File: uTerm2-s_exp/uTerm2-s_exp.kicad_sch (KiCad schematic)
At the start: 17 parts, among them J1 Conn_01x16_Female, J2 USB_B_Mini, J3 SD_Card, J4 Conn_01x08_Female, U1 ESP-PSRAM32, U2 CH340G, Y1 12MHz

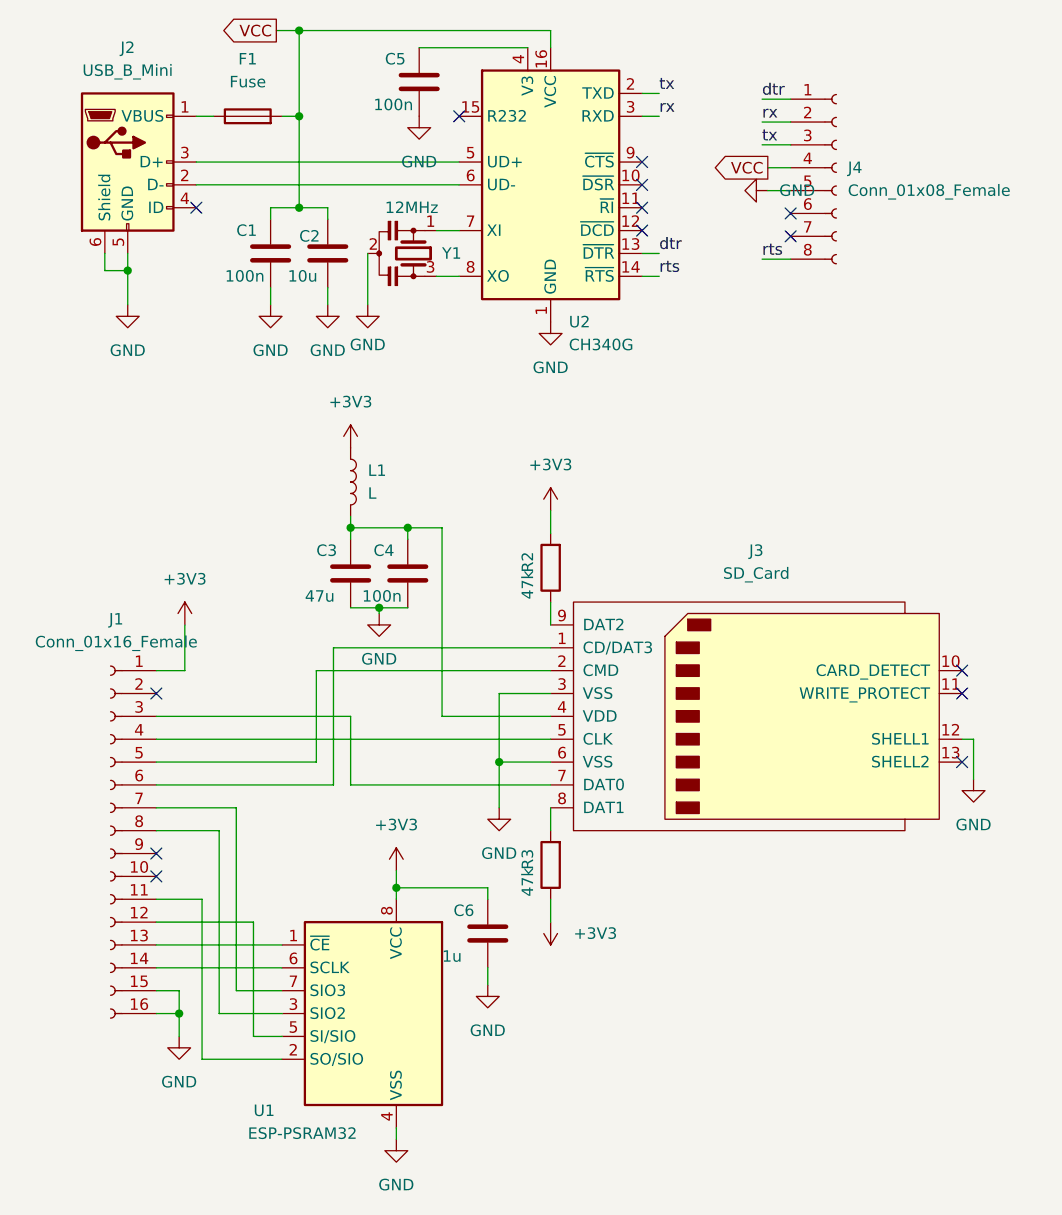
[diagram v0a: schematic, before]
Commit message: Signed-off-by: DamianPodrazaCode <damian.podraza@gmail.com>
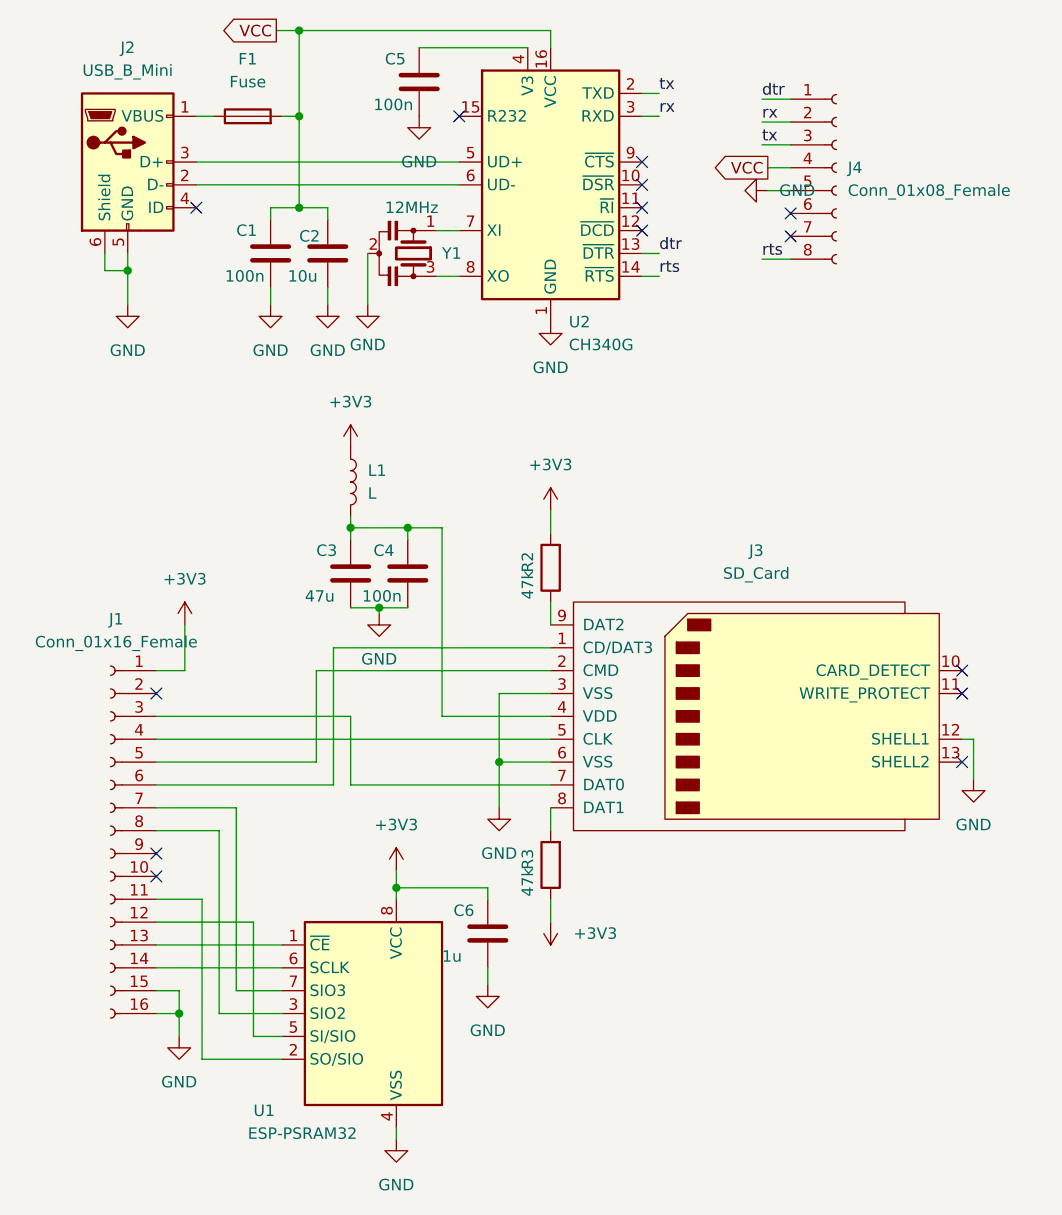
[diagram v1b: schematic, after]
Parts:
- J2: footprint (none) -> Connector_USB:USB_Mini-B_Lumberg_2486_01_Horizontal
